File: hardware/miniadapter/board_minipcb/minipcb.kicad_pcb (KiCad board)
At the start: 2 copper layers, 8.5 x 12.7 mm, 22 parts, among them Q102 FDG1024NZ, U102 SN74LVC1G14DRL, U103 TPS62933P

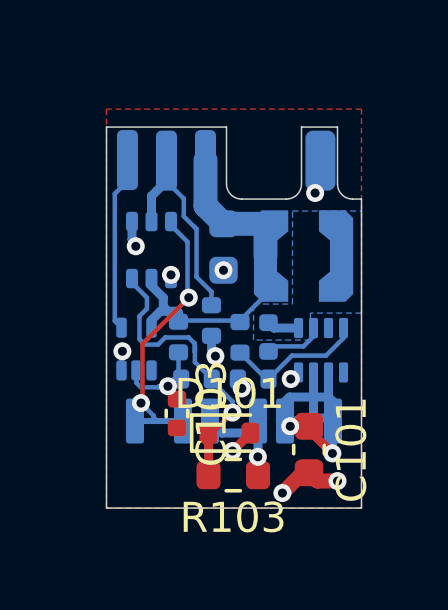
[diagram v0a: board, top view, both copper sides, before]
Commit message: new layout
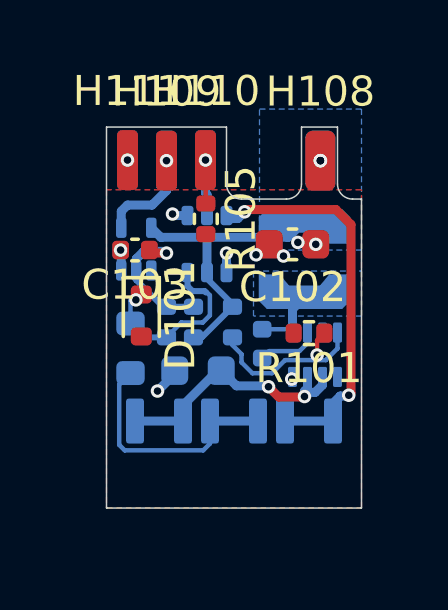
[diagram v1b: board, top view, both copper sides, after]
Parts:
- added H108: Pad, Connector_Wire:SolderWirePad_1x01_SMD_1.5x3mm, F.Cu at (107.1, 101.1)
- added H109: Pad, Connector_Wire:SolderWirePad_1x01_SMD_1.5x3mm, F.Cu at (102.0, 101.1)
- added H110: Pad, Connector_Wire:SolderWirePad_1x01_SMD_1.5x3mm, F.Cu at (103.3, 101.1)
- added H111: Pad, Connector_Wire:SolderWirePad_1x01_SMD_1.5x3mm, F.Cu at (100.7, 101.1)
- added REF**: Tab, PCM_kikit:Tab, F.Cu at (104.2, 112.7)
- added REF**: Tab, PCM_kikit:Tab, F.Cu at (108.5, 110.0)
- added REF**: Tab, PCM_kikit:Tab, F.Cu at (100.0, 102.0)
- C101, R103: moved to B.Cu
- C102, R101, R105: moved to F.Cu
- H101, H102, H103, H104, H105, H106, H107: value MountingHole_Pad -> Pad
- moved C103 5.63 mm to (101.0, 104.1), turned to 180 degrees
- moved R103 5.44 mm to (100.8, 107.4), turned to 90 degrees
- moved H101 5.00 mm to (101.8, 110.8)
- moved H103 5.00 mm to (106.8, 110.8)
- moved D101 4.90 mm to (101.2, 106.3), turned to -90 degrees
- moved C101 4.54 mm to (103.0, 108.1), turned to 180 degrees
- moved R105 3.40 mm to (103.3, 103.1)
- moved U102 3.33 mm to (101.0, 104.1)
- moved R101 2.41 mm to (106.8, 106.9)
- moved C102 2.30 mm to (106.2, 103.9), turned to 180 degrees
- moved R102 2.15 mm to (102.0, 106.5), turned to 90 degrees
- moved Q102 1.86 mm to (103.3, 103.9)
- moved R106 0.71 mm to (102.9, 106.5), turned to 90 degrees
- moved R104 0.57 mm to (104.2, 106.5)
- moved C104 0.30 mm to (105.2, 107.2)
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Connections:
- H104 pad 1: +3V3 -> /IO4
- H105 pad 1: /IO4 -> /IO5
- H106 pad 1: GND -> +3V3
- H107 pad 1: /IO5 -> GND
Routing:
- net /IO4: track 7.79 -> 3.32 mm, vias 0 -> 1
- net /DBUS: track 3.73 -> 8.09 mm, vias 1 -> 0
- net /DBUS_R: track 10.2 -> 6.22 mm
- net GND: track 8.01 -> 4.10 mm, vias 11 -> 8
- net /V-: track 9.38 -> 13.1 mm
- net /IO5: track 5.86 -> 3.34 mm, vias 0 -> 1
- net +3V3: track 12.4 -> 10.5 mm, vias 0 -> 4
- net /V+: track 10.2 -> 8.75 mm
- net /SW: track 1.07 -> 2.40 mm
- net /FB: track 4.83 -> 6.01 mm, vias 0 -> 1
- net /IN: track 3.79 -> 4.73 mm
- added copper zone on B.Cu, net +3V3
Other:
- board text added: "3V3"
- board text added: "GND"
- board text added: "IO4"
- board text added: "IO5"
